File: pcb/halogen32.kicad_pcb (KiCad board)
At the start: 2 copper layers, 41 parts, among them J1 Conn_ARM_JTAG_SWD_10, J2 USB_C_Receptacle_USB2.0_16P, J3 Conn_01x04_Pin, J4 Conn_01x20_Socket, J5 Conn_01x14_Socket, J6 Barrel_Jack, SW1 SW_SPDT, SW2 SW_SPDT, U1 STM32F411CEUx, U2 AMS1117-3.3, U3 LM2576HVS-5, Y1 16MHz

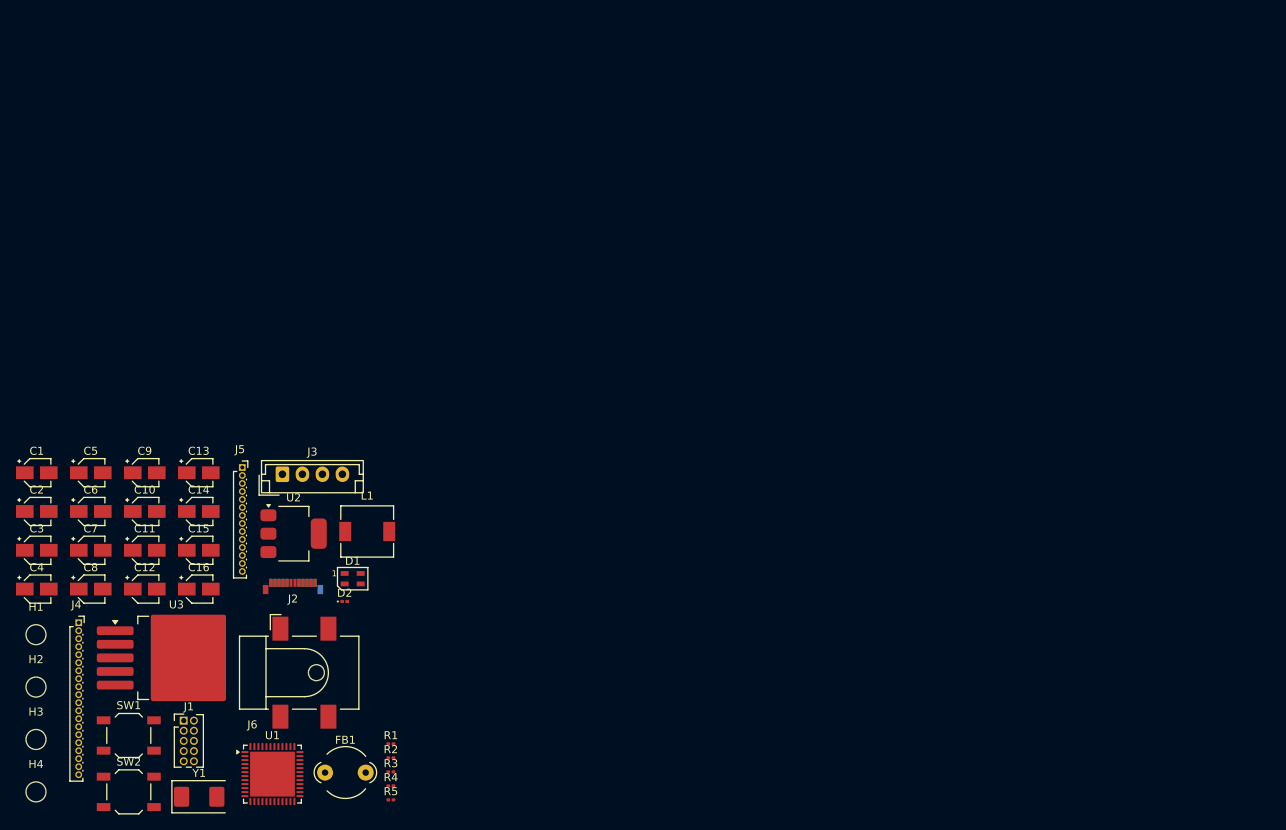
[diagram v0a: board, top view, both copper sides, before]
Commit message: Began work on rough layout.
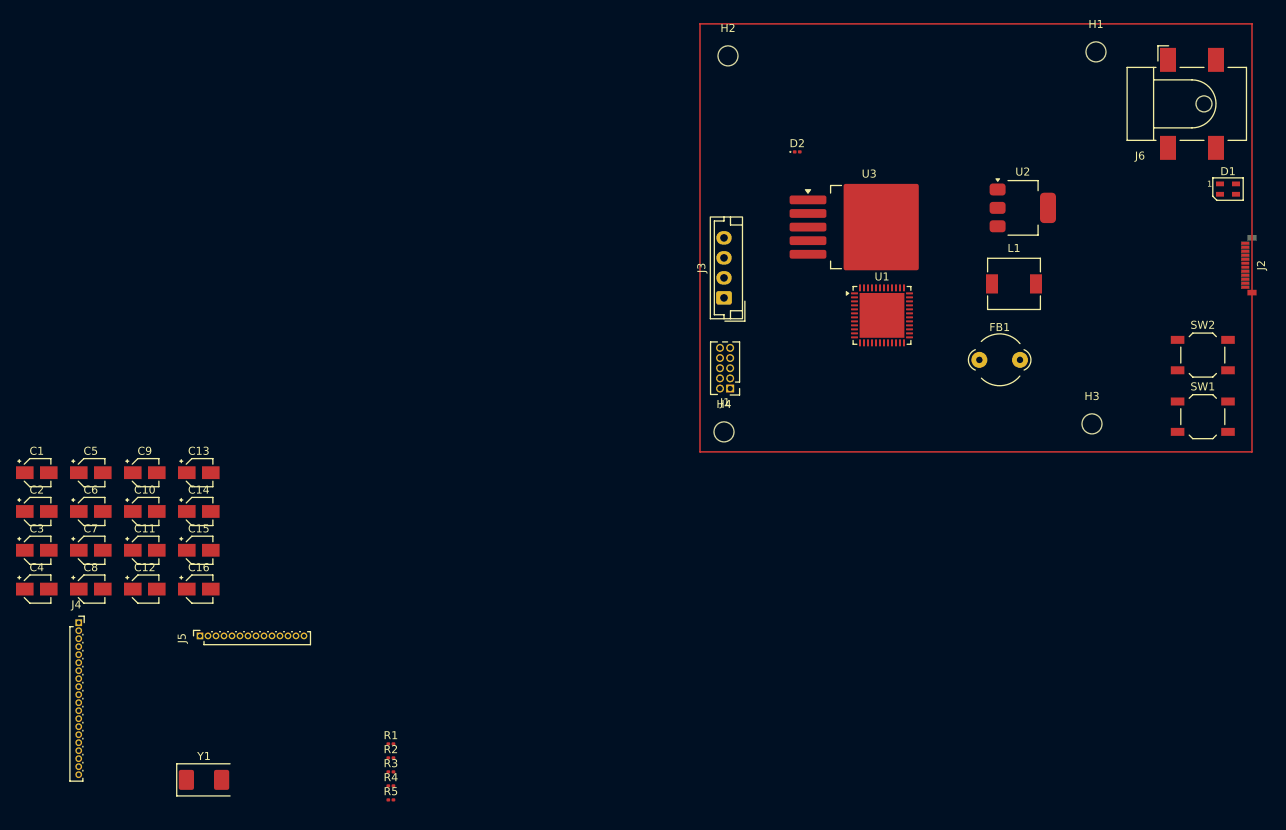
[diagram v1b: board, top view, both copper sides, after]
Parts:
- moved H1 151.2 mm to (151.0, 98.0)
- moved SW2 144.9 mm to (164.3, 135.9)
- moved SW1 140.0 mm to (164.3, 143.6)
- moved H3 137.8 mm to (150.5, 144.5)
- moved J6 131.8 mm to (163.0, 104.5)
- moved J2 125.4 mm to (169.6, 124.7), turned to 90 degrees
- moved D1 119.8 mm to (167.5, 115.2)
- moved H2 117.1 mm to (105.0, 98.5)
- moved U3 102.0 mm to (122.7, 119.9)
- moved U2 99.8 mm to (141.8, 117.5)
- moved H4 97.1 mm to (104.5, 145.5)
- moved FB1 96.7 mm to (136.4, 136.5)
- moved U1 95.4 mm to (124.2, 130.9)
- moved L1 86.6 mm to (140.8, 127.0)
- moved J1 79.9 mm to (105.3, 140.1), turned to 180 degrees
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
